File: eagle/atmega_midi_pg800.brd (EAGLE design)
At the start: 101 x 81 mm, 19 parts, among them IC1 78L05Z, U1 6N138, U2 ATMEGA328P_PDIP, X1 MAB6H

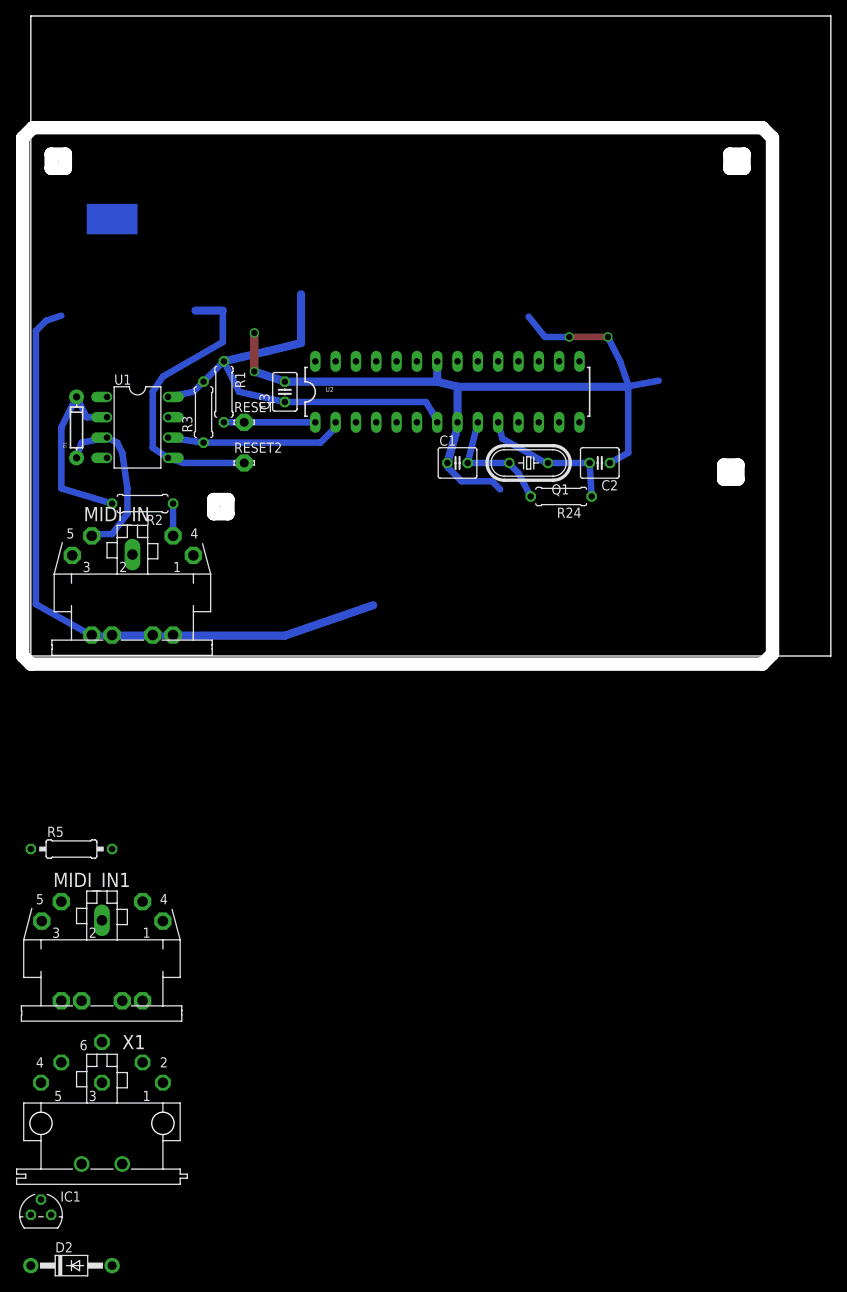
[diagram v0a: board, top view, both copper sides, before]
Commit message: routed
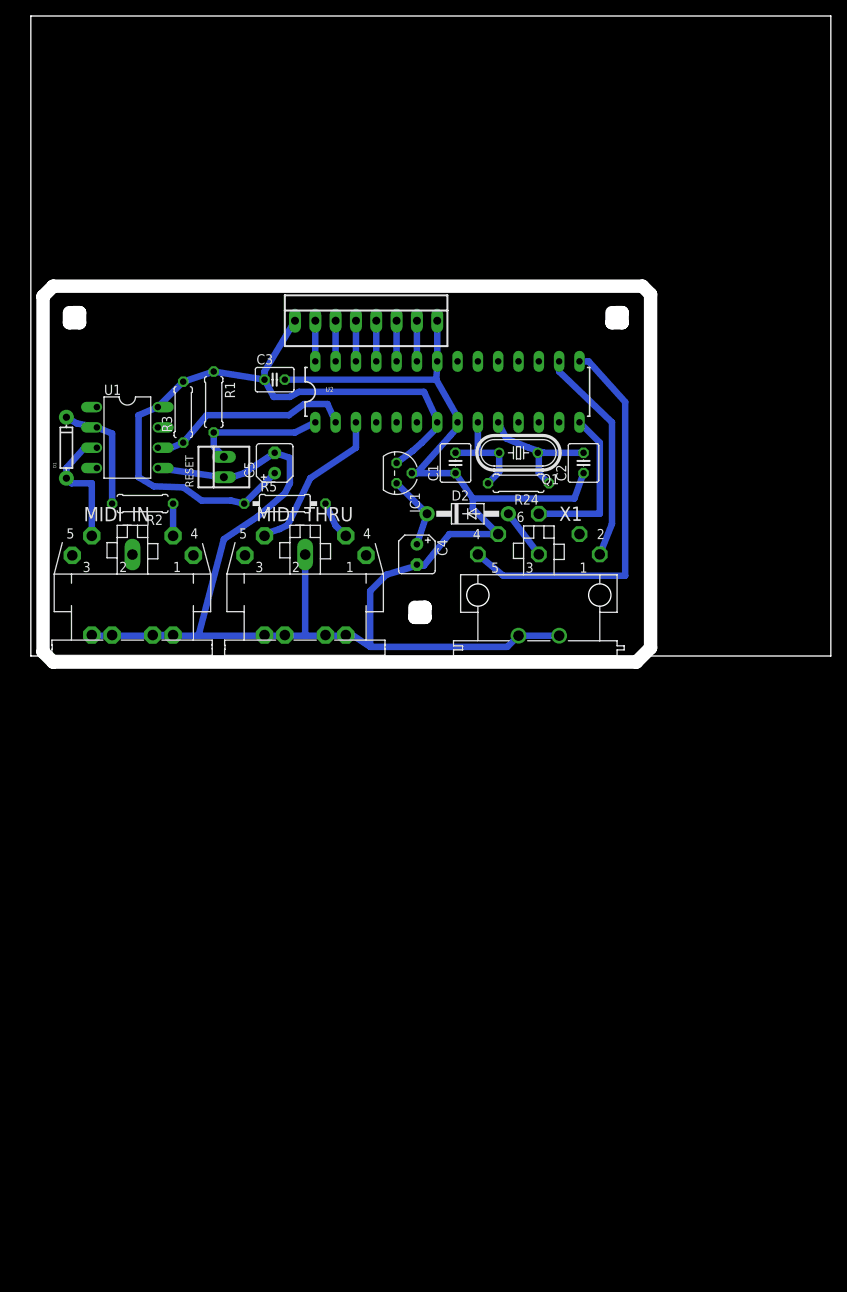
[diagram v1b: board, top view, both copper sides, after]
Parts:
- removed MIDI_IN1: MIDIJACK, adafruit:CP-2350
- removed RESET2: LSP11, solpad:LSP11
- added C4: 100uF, rcl:B45181A
- added C5: 10uF, rcl:B45181A
- added MIDI_THRU: MIDIJACK, adafruit:CP-2350
- added X2: 22-23-2081, con-molex:22-23-2081
- RESET: value LSP11 -> 22-23-2021; device solpad:LSP11 -> con-molex:22-23-2021
- moved D2 106.2 mm to (54.6, 17.8)
- moved IC1 102.8 mm to (45.7, 22.9), turned to 270 degrees
- moved X1 85.7 mm to (63.5, 7.62)
- moved R5 50.8 mm to (31.8, 19.1)
- moved RESET 6.14 mm to (24.1, 23.6), turned to 90 degrees
- moved R24 5.58 mm to (61.0, 21.6)
- moved D1 2.84 mm to (4.45, 26.0)
- moved R3 2.54 mm to (19.1, 30.5)
- moved C2 2.03 mm to (69.1, 24.1), turned to 90 degrees
- moved C3 1.98 mm to (30.5, 34.5), turned to 0 degrees
- moved R1 1.80 mm to (22.9, 31.8)
- moved U1 1.80 mm to (12.1, 27.3)
- moved Q1 1.80 mm to (61.0, 25.4)
- moved C1 0.25 mm to (53.1, 24.1), turned to 90 degrees
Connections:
- removed net PE: X1.PE, X1.PE@
- new net N$10: U2.16, X1.1
- new net N$11: U2.15, X1.5
- new net N$12: U2.23, X2.7
- new net N$13: U2.24, X2.6
- new net N$14: U2.25, X2.5
- new net N$15: U2.26, X2.4
- new net N$16: U2.27, X2.3
- new net N$17: U2.28, X2.2
- new net N$2: D2.A, X1.3
- new net N$6: C4.+, D2.C, IC1.3
- new net N$9: U2.14, X1.6
- net +5V: now also C5.+, IC1.1, X2.1
- net GND: now also C4.-, C5.-, IC1.2, MIDI_THRU.2, MIDI_THRU.PE, MIDI_THRU.PE1, MIDI_THRU.PE2, MIDI_THRU.PE@, RESET.1, X1.4, X1.PE, X1.PE@, X2.8; no longer MIDI_IN1.2, MIDI_IN1.PE, MIDI_IN1.PE1, MIDI_IN1.PE2, MIDI_IN1.PE@, RESET2.MP
- net N$1: now also MIDI_THRU.4; no longer MIDI_IN1.4
- net N$42: now also MIDI_THRU.5; no longer MIDI_IN1.5
- net N$43: now also RESET.2; no longer RESET.MP
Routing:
- net N$11: track 0.00 -> 49.1 mm
- net +5V: track 55.3 -> 86.3 mm
- net N$10: track 0.00 -> 27.2 mm
- net N$9: track 0.00 -> 20.1 mm
- net N$42: track 0.00 -> 19.9 mm
- net GND: track 226.8 -> 215.6 mm, vias 4 -> 0
- net N$6: track 0.00 -> 9.40 mm
- net N$7: track 23.9 -> 14.9 mm
- net N$2: track 0.00 -> 6.35 mm
- net N$3: track 21.7 -> 16.2 mm
- net N$43: track 11.4 -> 16.6 mm
- net N$17: track 0.00 -> 5.08 mm
- net N$16: track 0.00 -> 5.08 mm
- net N$15: track 0.00 -> 5.08 mm
- net N$14: track 0.00 -> 5.08 mm
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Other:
- board size 101 x 81 mm -> 100 x 80.8 mm

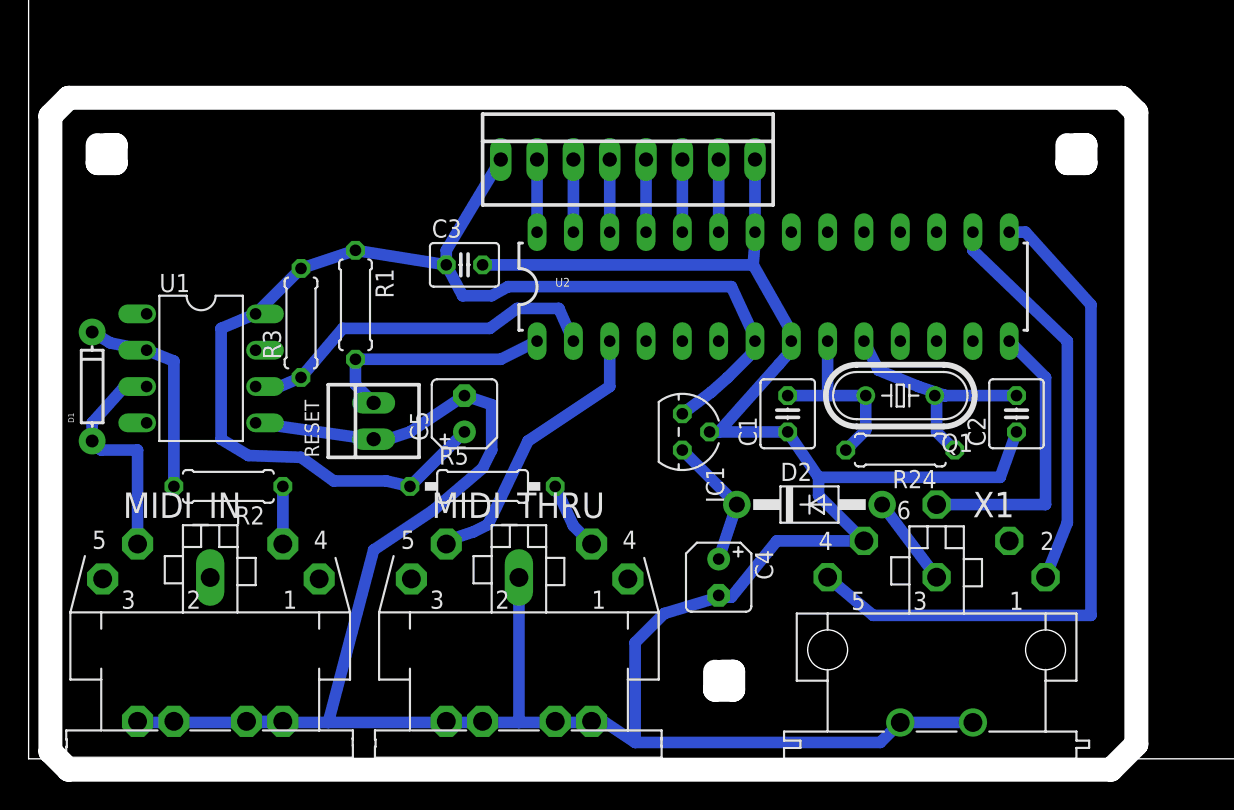
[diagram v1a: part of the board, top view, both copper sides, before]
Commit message: gcode
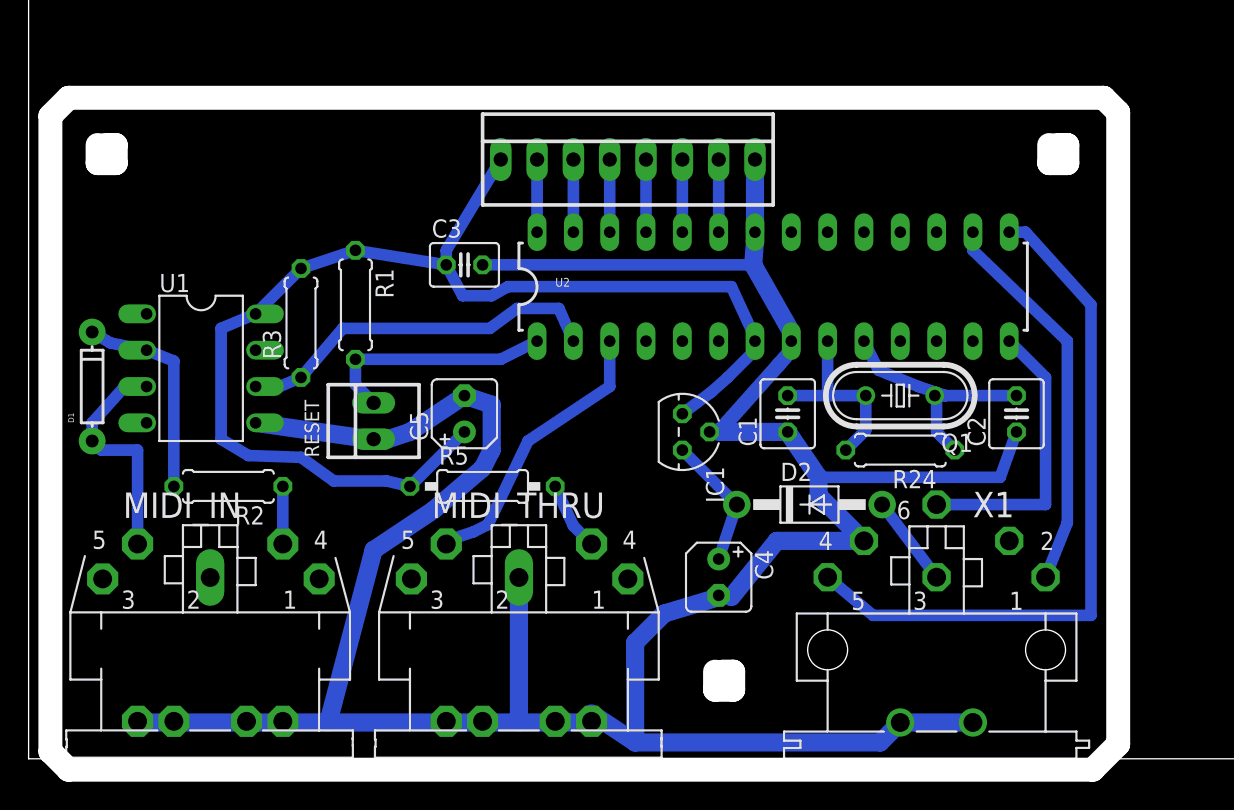
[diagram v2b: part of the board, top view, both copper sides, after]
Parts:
- Q1: value (none) -> 16.000Mhz
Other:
- outline, holes or cut-outs redrawn
